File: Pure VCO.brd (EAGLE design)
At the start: 48.8 x 100 mm, 104 parts, among them IC1 TL072D, IC2 TL072D, IC3 TL072D, IC4 TL072D, IC5 TL072D, IC6 TL072D, J1 S_JACK, J2 S_JACK, J3 S_JACK, J4 S_JACK, J5 S_JACK, J6 S_JACK, J7 S_JACK, J8 S_JACK, T1 N_CHN, U1 LM4040A50IDBZT

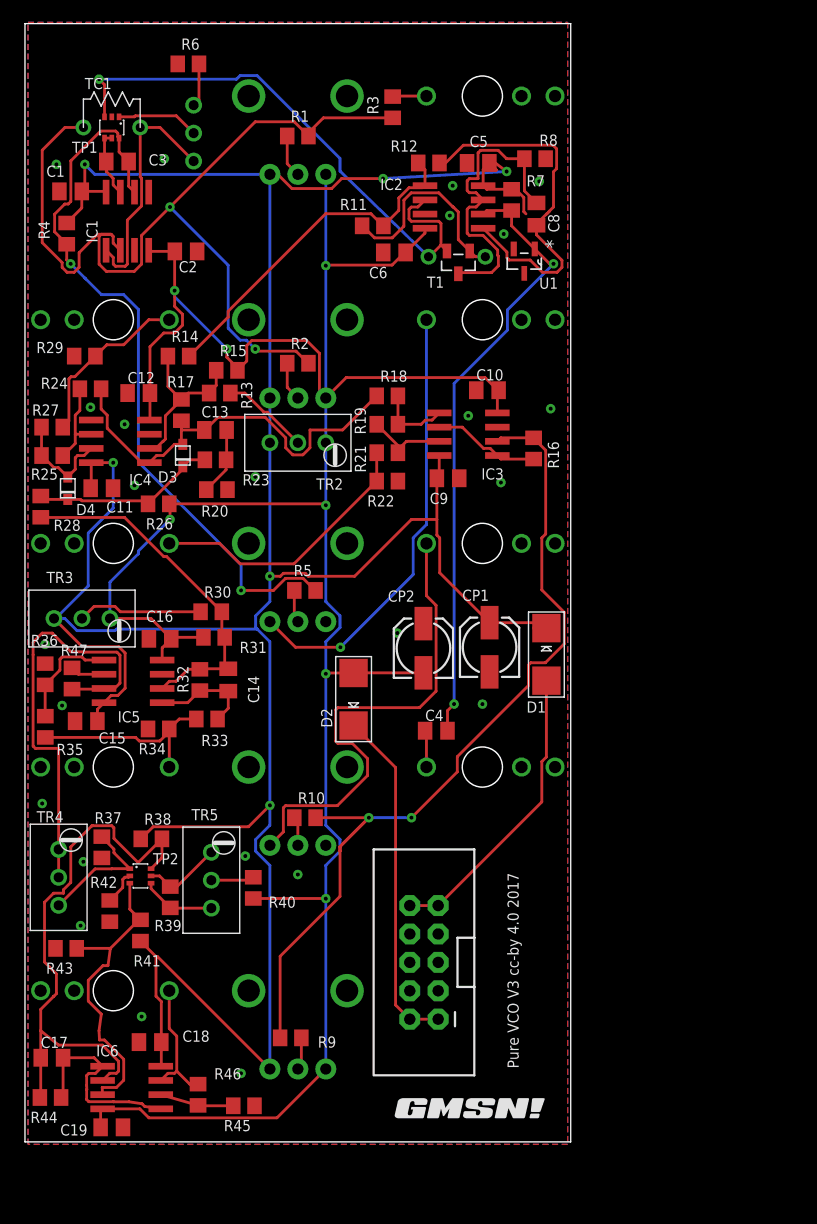
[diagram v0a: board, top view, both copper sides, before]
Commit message: VCO 3.0
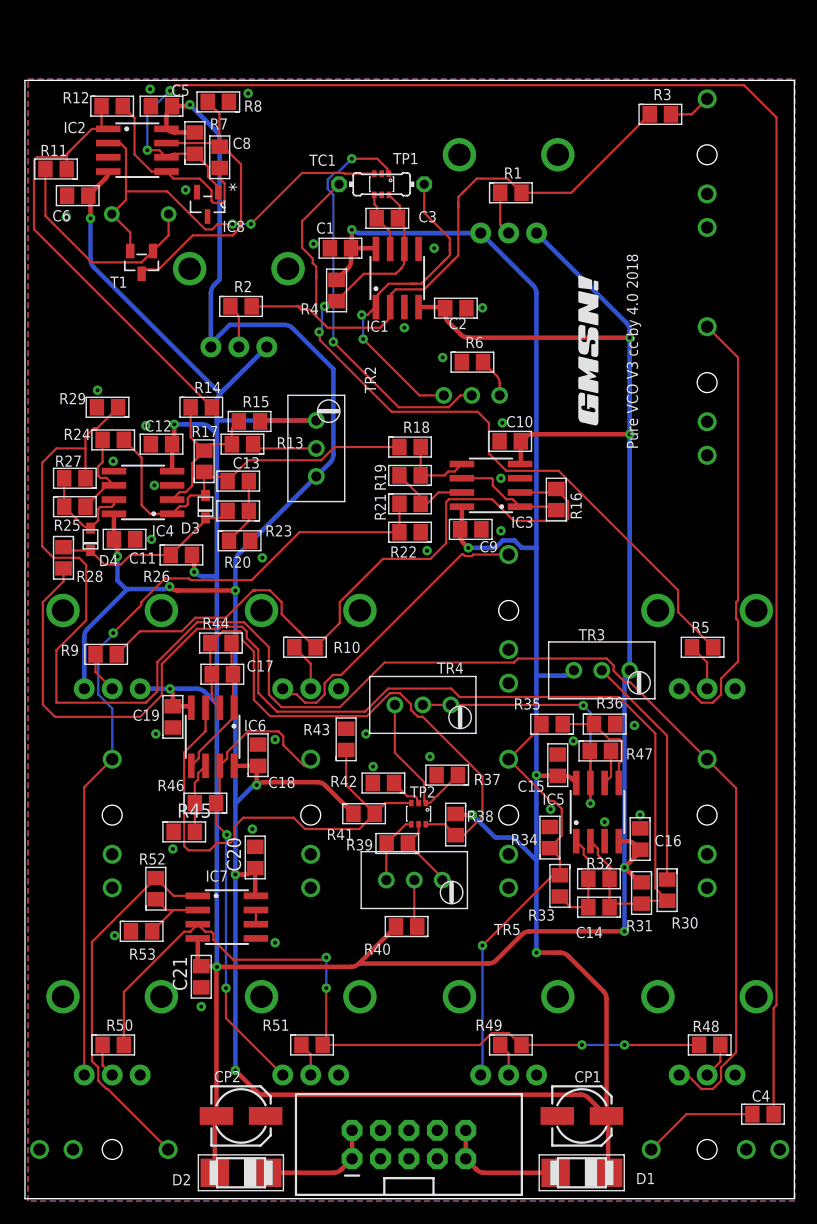
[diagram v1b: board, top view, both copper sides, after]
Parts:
- removed J1, J2, J3, J4, J5, J6, J7, J8: S_JACK, GMSN:S_JACK
- removed U1: LM4040A50IDBZT, GMSN:SOT95P237X112-3N
- removed VR1: Coarse, GMSN:POT
- removed VR2, VR3, VR4, VR5: B100K, GMSN:POT
- added 1V/OCT, LIN, MIX, PULSE, PWM_IN, SAW, SINE, SYNC, TRI: PJ301M-12, GMSN:PJ301M-12
- added C20, C21: 100nF, GMSN:C0805
- added COARSE, FINE, FM_LEVEL, PULSE_MIX, PULSE_WIDTH, PWM_LEVEL, SAW_MIX, SINE_MIX, TRI_MIX: B100k, GMSN:POTENTIOMETER_9MM
- added IC7: TL072, GMSN:SO08
- added IC8: LM4040A50IDBZT, GMSN:SOT95P237X112-3N
- added R48, R49, R50, R51, R52, R53: 100k, GMSN:R0805
- C1, C10, C11, C12, C15, C16, C18, C19, C2, C5, C6, C9: value 100n -> 100nF; device GMSN:C0805K -> GMSN:C0805
- C13: device GMSN:C0805K -> GMSN:C0805
- C14: value 1000p -> 1nF; device GMSN:C0805K -> GMSN:C0805
- C17, C3, C4: value 100p -> 100pF; device GMSN:C0805K -> GMSN:C0805
- C7: value 2.2n -> 2.2nF
- C8: value 22p -> 22pF; device GMSN:C0805K -> GMSN:C0805
- CP1, CP2: value 10u -> 10uF
- D1, D2: value (none) -> STTH102A
- D3, D4: value (none) -> 1N914
- IC1, IC2, IC3, IC4, IC5, IC6: value TL072D -> TL072
- JP1: value M05X2SHD -> HEADER2X5SHD; device SparkFun-Connectors:2X5-SHROUDED -> GMSN:2X5-SHROUDED
- R1: value 150K -> 150k
- R10, R17: value 39K -> 39k
- R12: value 9K1 -> 9k1
- R13: value 5K6 -> 5k6
- R14, R20, R23, R28, R38, R40, R41, R43, R44: value 10K -> 10k
- R15: value 56K -> 56k
- R16, R3, R30: value 100K -> 100k
- R18: value 2K2 -> 2k2
- R21: value 3K3 -> 1k5
- R22: value 1K5 -> 1k5
- R24, R25: value 22K* -> 22k
- R27, R29, R34, R37, R42: value 2K -> 2k
- R31: value 27K -> 27k
- R32, R46: value 10K -> 19k1
- R33, R35, R47: value 1K3 -> 1k3
- R36, R8: value 3K3 -> 3k3
- R45: value empty -> 10k
- R5: value 560K -> 560k
- R9: value 120K -> 120k
- T1: value N_CHN -> MMBFJ309
- TC1: value 2K -> 2k; device GMSN:RESISTOR_TC -> GMSN:0204/7
- TP1, TP2: value TRANS_PAIR -> DMMT3904W-7-F
- TR1: device GMSN:TRIMMER_TH3 -> GMSN:TRIMMER_TH
- TR2, TR3, TR4, TR5: value 100K -> 100k; device GMSN:TRIMMER_TH3 -> GMSN:TRIMMER_TH
- moved U$1 68.9 mm to (51.5, 87.8), turned to 90 degrees
- moved R36 50.2 mm to (52.8, 54.1), turned to 0 degrees
- moved TR3 50.1 mm to (55.9, 57.8)
- moved R30 47.8 mm to (58.4, 39.2), turned to 270 degrees
- moved R47 47.7 mm to (52.5, 51.7), turned to 0 degrees
- moved C16 46.5 mm to (56.0, 43.8), turned to 270 degrees
- moved D1 46.5 mm to (50.8, 14.0), turned to 180 degrees
- moved R35 45.3 mm to (48.1, 54.1), turned to 180 degrees
- moved C4 45.0 mm to (67.0, 19.2)
- moved CP2 44.9 mm to (20.3, 19.1), turned to 0 degrees
- moved R31 44.5 mm to (56.1, 39.0), turned to 270 degrees
- moved D2 43.5 mm to (20.3, 14.0), turned to 180 degrees
- moved R44 43.4 mm to (18.5, 61.3)
- moved IC5 43.1 mm to (52.2, 46.2), turned to 0 degrees
- moved CP1 42.7 mm to (50.8, 19.1), turned to 0 degrees
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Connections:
- removed net N$27: J6.TIP, R27.1, R29.1
- new net N$25: IC7.6, IC7.7
- new net N$35: IC7.3, R48.2, R49.2, R50.2, R51.2
- new net N$38: R48.1, SAW_MIX.P$2
- new net N$43: R49.1, TRI_MIX.P$2
- new net N$45: R51.1, SINE_MIX.P$2
- new net N$48: IC7.2, R52.1, R53.2
- new net N$49: IC7.1, MIX.TIP, R52.2
- new net PULSE: PULSE.TIP, PULSE_MIX.P$3, R21.1, R22.2
- new net SAW: R27.1, R29.1, SAW.TIP, SAW_MIX.P$3
- net +12V: now also C20.1, COARSE.P$3, FINE.P$3, IC7.8, PULSE_WIDTH.P$3; no longer VR1.P$3, VR2.P$3, VR4.P$3
- net -12V: now also C21.2, COARSE.P$1, FINE.P$1, IC7.4, PULSE_WIDTH.P$1; no longer VR1.P$1, VR2.P$1, VR4.P$1
- net GND: now also 1V/OCT.GND, 1V/OCT.NORM, C20.2, C21.1, FM_LEVEL.P$1, IC7.5, IC8.2, LIN.GND, LIN.NORM, MIX.GND, PULSE.GND, PULSE_MIX.P$1, PWM_IN.GND, PWM_LEVEL.P$1, R53.1, SAW.GND, SAW_MIX.P$1, SINE.GND, SINE_MIX.P$1, SYNC.GND, TRI.GND, TRI_MIX.P$1; no longer J1.GND, J1.NORM, J2.GND, J2.NORM, J3.GND, J4.GND, J5.GND, J6.GND, J7.GND, J8.GND, U1.2, VR3.P$1, VR5.P$1
- net N$15: now also FM_LEVEL.P$3, LIN.TIP; no longer J1.TIP, VR3.P$3
- net N$17: now also FM_LEVEL.P$2; no longer VR3.P$2
- net N$2: now also COARSE.P$2; no longer VR1.P$2
- net N$21: now also SYNC.TIP; no longer J3.TIP
- net N$22: now also IC8.1; no longer U1.1
- net N$40: now also PULSE_WIDTH.P$2; no longer VR4.P$2
- net N$41: now also PWM_IN.TIP, PWM_LEVEL.P$3; no longer J4.TIP, VR5.P$3
- net N$44: now also PULSE_MIX.P$2, R50.1; no longer J5.TIP, R21.1, R22.2
- net N$46: now also PWM_LEVEL.P$2; no longer VR5.P$2
- net N$5: now also FINE.P$2; no longer VR2.P$2
- net N$9: now also 1V/OCT.TIP; no longer J2.TIP
- net SINE: now also SINE.TIP, SINE_MIX.P$3; no longer J8.TIP
- net TRI: now also TRI.TIP, TRI_MIX.P$3; no longer J7.TIP
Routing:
- net SAW: track 0.00 -> 146.8 mm
- net N$22: track 54.9 -> 159.9 mm
- net N$34: track 31.7 -> 108.8 mm
- net PULSE: track 0.00 -> 73.9 mm, vias 0 -> 1
- net N$35: track 0.00 -> 69.4 mm, vias 0 -> 4
- net -12V: track 231.3 -> 288.5 mm, vias 7 -> 9
- net +12V: track 273.7 -> 327.5 mm, vias 6 -> 12
- net N$49: track 0.00 -> 33.9 mm
- net SINE: track 11.6 -> 42.1 mm, vias 0 -> 2
- net N$10: track 7.35 -> 36.9 mm, vias 0 -> 2
- net N$44: track 24.9 -> 3.04 mm
- net TRI: track 17.8 -> 38.9 mm, vias 0 -> 1
- net N$3: track 30.9 -> 10.6 mm
- net N$42: track 80.6 -> 61.9 mm, vias 2 -> 0
- net N$4: track 84.4 -> 66.0 mm, vias 2 -> 0
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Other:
- board size 48.8 x 100 mm -> 68.8 x 100 mm
- board text added: "Pure VCO V3 cc-by 4.0 2018"
- board text removed: "Pure VCO V3 cc-by 4.0 2017"
